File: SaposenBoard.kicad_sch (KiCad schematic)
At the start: 66 parts, among them IC1 BSO220, IC2 BSO220, IC3 BSO220, IC4 BSO220, J1 ADC4ch, J2 Extra2ch+LED, J3 Encoder1, J4 Encoder2, J5 I2C, J6 Battery, J7 Motor1, J8 Motor2, Q2 IRLML6344, SW1 BatterySW, SW2 SW_Push, SW3 SW_Push, U1 A4955GLPTR-T, U2 A4955GLPTR-T, U3 MPU-6500, U4 NUCLEO-F303K8

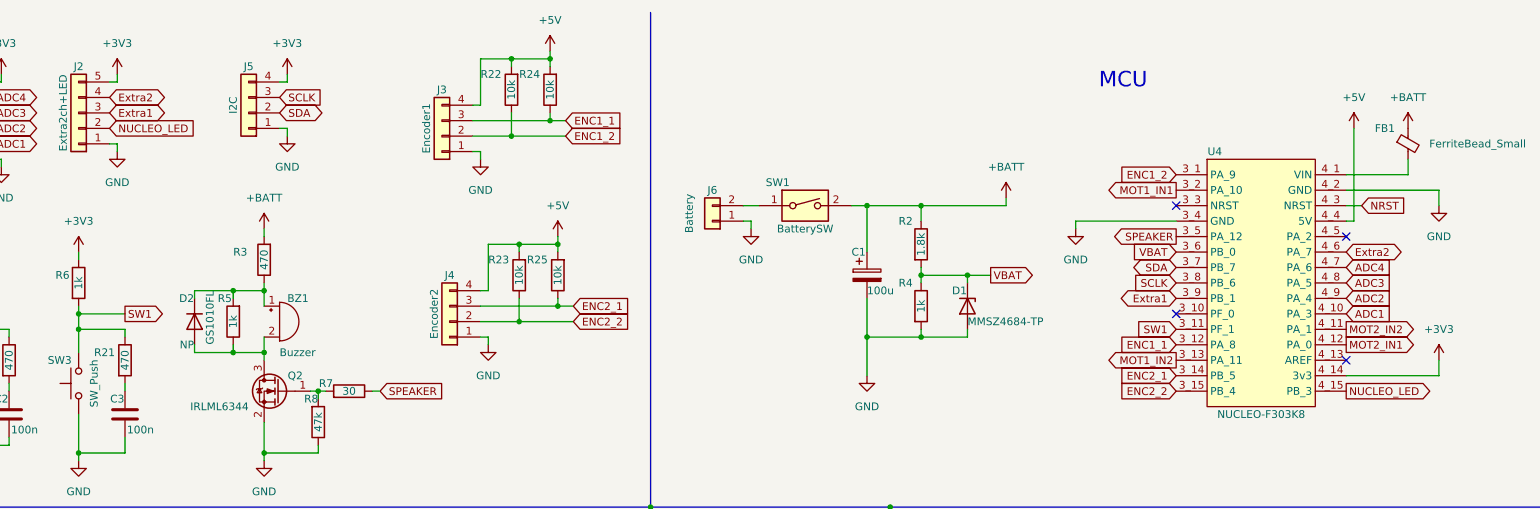
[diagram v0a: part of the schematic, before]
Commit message: [update]終わった
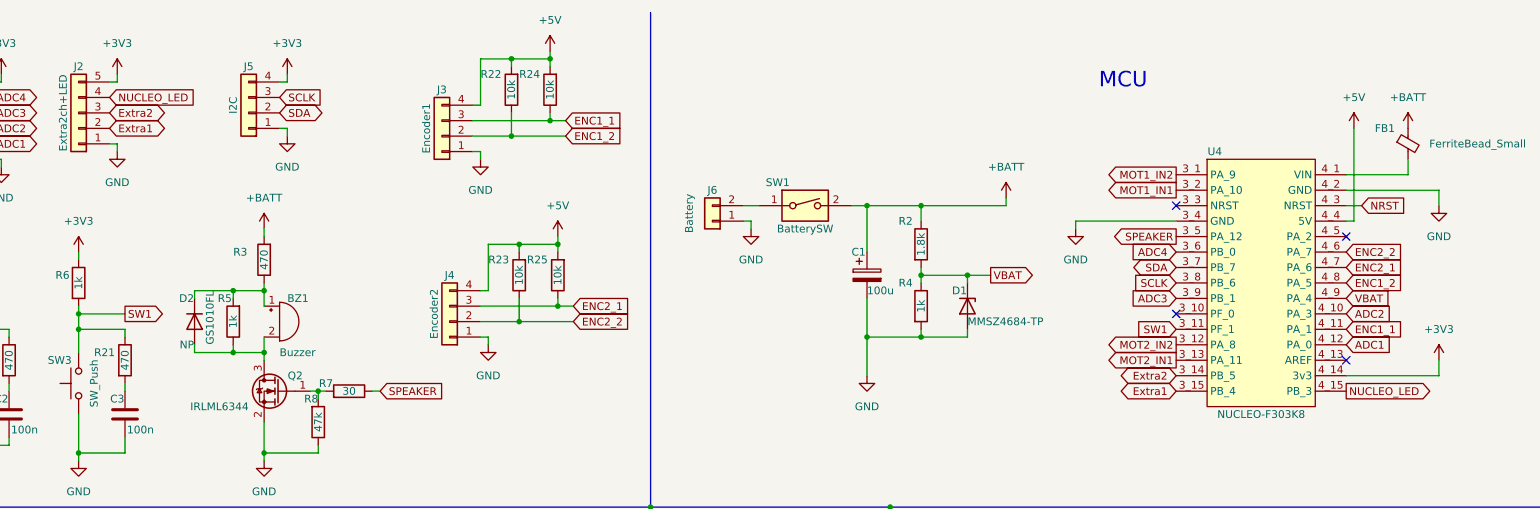
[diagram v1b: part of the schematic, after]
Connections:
- net ADC1: now also U4.4_12 (PA_0); no longer U4.4_10 (PA_3)
- net ADC2: now also U4.4_10 (PA_3); no longer U4.4_9 (PA_4)
- net ADC3: now also U4.3_9 (PB_1); no longer U4.4_8 (PA_5)
- net ADC4: now also U4.3_6 (PB_0); no longer U4.4_7 (PA_6)
- net ENC1_1: now also U4.4_11 (PA_1); no longer U4.3_12 (PA_8)
- net ENC1_2: now also U4.4_8 (PA_5); no longer U4.3_1 (PA_9)
- net ENC2_1: now also U4.4_7 (PA_6); no longer U4.3_14 (PB_5)
- net ENC2_2: now also U4.4_6 (PA_7); no longer U4.3_15 (PB_4)
- net Extra1: now also J2.2 (Pin_2), U4.3_15 (PB_4); no longer J2.3 (Pin_3), U4.3_9 (PB_1)
- net Extra2: now also J2.3 (Pin_3), U4.3_14 (PB_5); no longer J2.4 (Pin_4), U4.4_6 (PA_7)
- net MOT1_IN2: now also U4.3_1 (PA_9); no longer U4.3_13 (PA_11)
- net MOT2_IN1: now also U4.3_13 (PA_11); no longer U4.4_12 (PA_0)
- net MOT2_IN2: now also U4.3_12 (PA_8); no longer U4.4_11 (PA_1)
- net NUCLEO_LED: now also J2.4 (Pin_4); no longer J2.2 (Pin_2)
- net VBAT: now also U4.4_9 (PA_4); no longer U4.3_6 (PB_0)

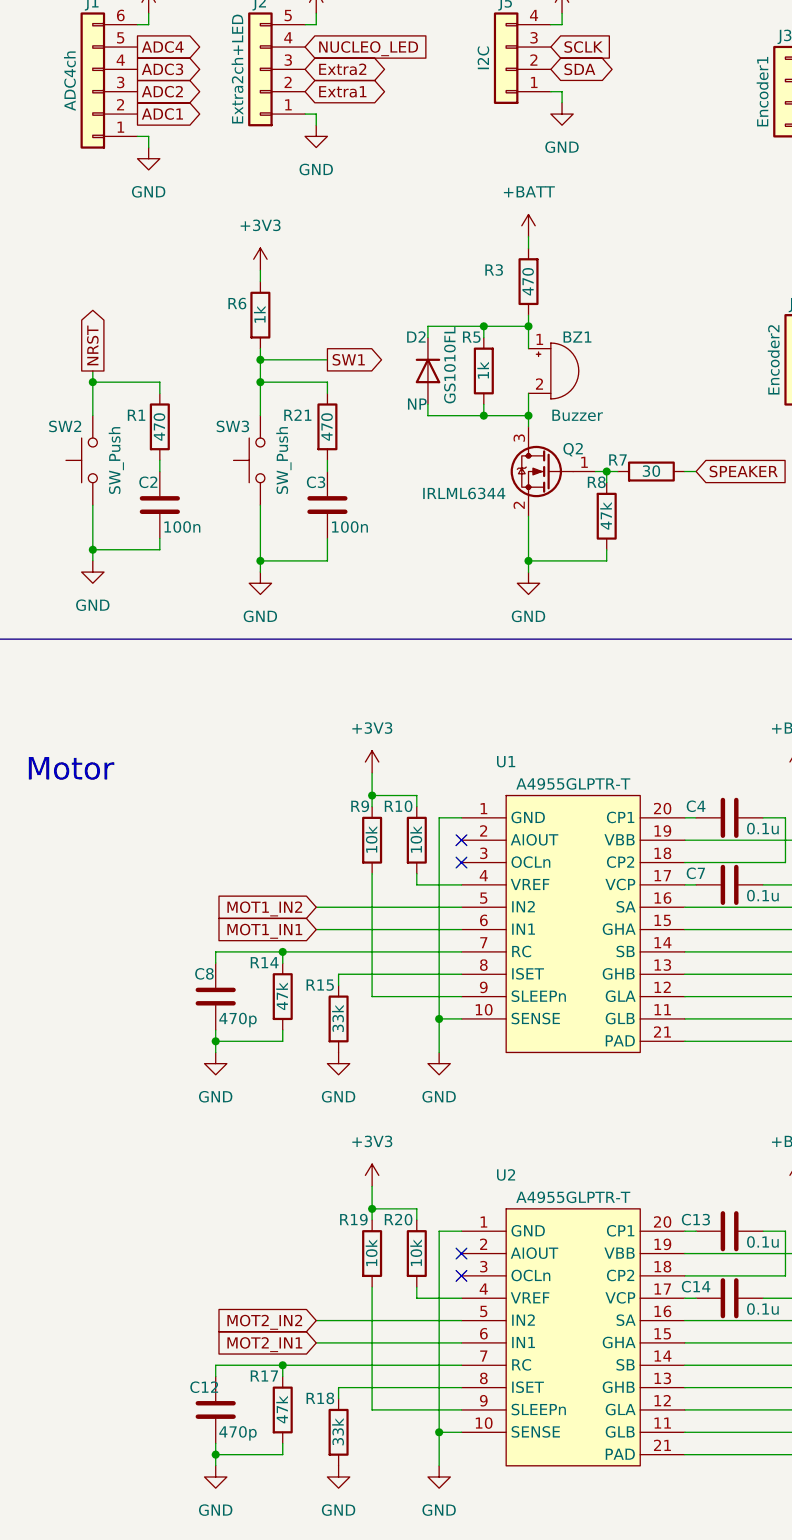
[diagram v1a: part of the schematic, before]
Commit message: a
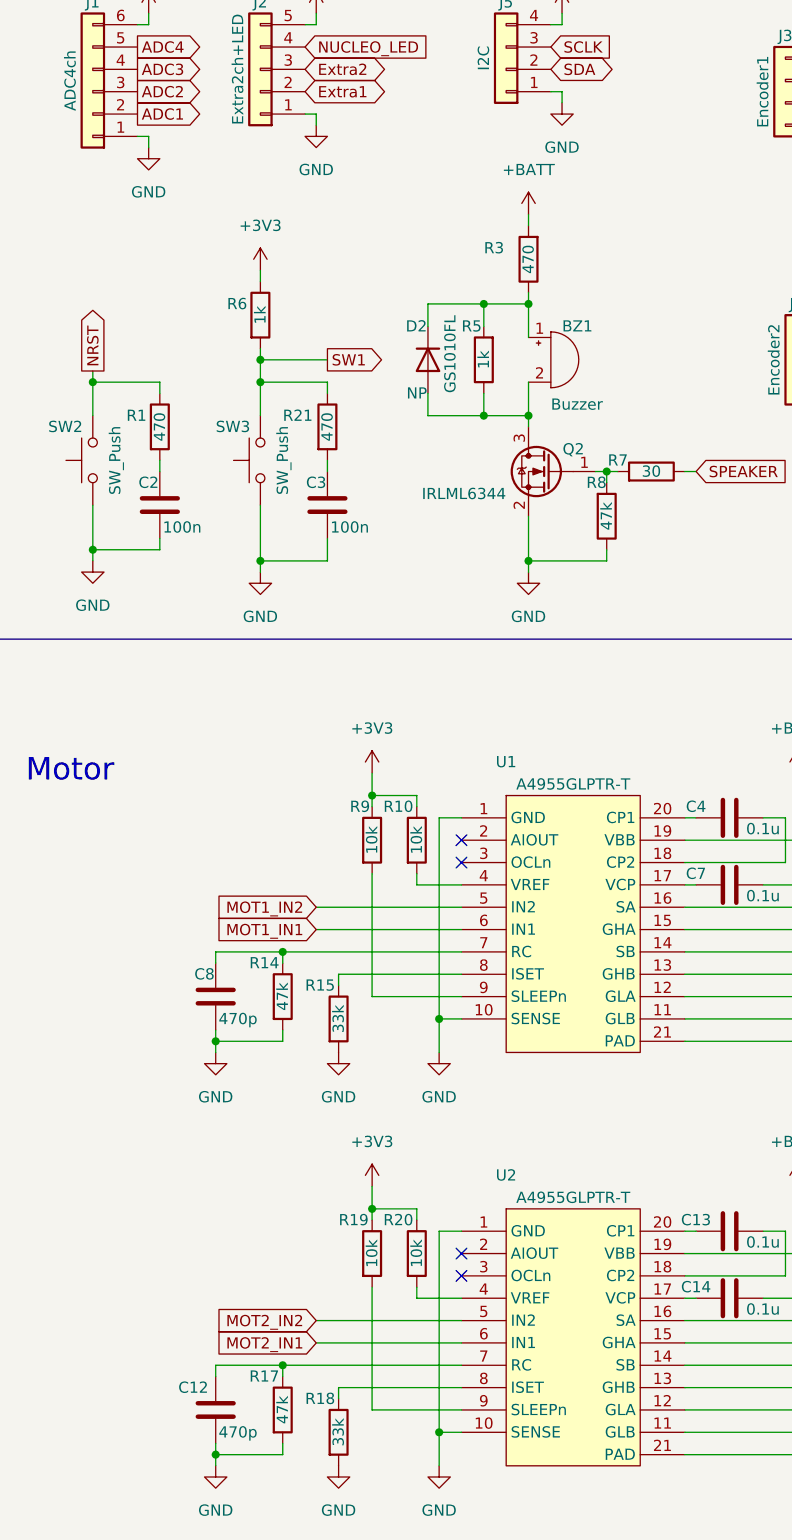
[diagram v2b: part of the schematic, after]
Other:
- moved on the sheet: BZ1, D2, R3, R5
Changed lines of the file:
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@@
   (junction (at 121.92 60.96) (diameter 0) (color 0 0 0 0)
   )
-  (junction (at 73.66 58.42) (diameter 0) (color 0 0 0 0)
+  (junction (at 73.66 55.88) (diameter 0) (color 0 0 0 0)
   )
   (junction (at 148.59 171.45) (diameter 0) (color 0 0 0 0)
@@
   (junction (at 38.1 139.7) (diameter 0) (color 0 0 0 0)
   )
+  (junction (at 68.58 55.88) (diameter 0) (color 0 0 0 0)
+  )
   (junction (at 55.88 111.76) (diameter 0) (color 0 0 0 0)
   )
@@
   )
   (junction (at 120.65 30.48) (diameter 0) (color 0 0 0 0)
-  )
-  (junction (at 68.58 58.42) (diameter 0) (color 0 0 0 0)
   )
   (junction (at 115.57 63.5) (diameter 0) (color 0 0 0 0)
@@
     (stroke (width 0) (type default) (color 0 0 0 0))
   )
-  (wire (pts (xy 62.23 67.31) (xy 62.23 68.58))
+  (wire (pts (xy 62.23 66.04) (xy 62.23 68.58))
     (stroke (width 0) (type default) (color 0 0 0 0))
   )
@@
     (stroke (width 0) (type default) (color 0 0 0 0))
   )
-  (wire (pts (xy 62.23 58.42) (xy 68.58 58.42))
+  (wire (pts (xy 62.23 55.88) (xy 68.58 55.88))
     (stroke (width 0) (type default) (color 0 0 0 0))
   )
@@
     (stroke (width 0) (type default) (color 0 0 0 0))
   )
-  (wire (pts (xy 73.66 57.15) (xy 73.66 58.42))
+  (wire (pts (xy 73.66 54.61) (xy 73.66 55.88))
     (stroke (width 0) (type default) (color 0 0 0 0))
   )
@@
     (stroke (width 0) (type default) (color 0 0 0 0))
   )
-  (wire (pts (xy 73.66 66.04) (xy 73.66 68.58))
+  (wire (pts (xy 73.66 64.77) (xy 73.66 68.58))
     (stroke (width 0) (type default) (color 0 0 0 0))
   )
@@
     (stroke (width 0) (type default) (color 0 0 0 0))
   )
+  (wire (pts (xy 68.58 55.88) (xy 68.58 58.42))
+    (stroke (width 0) (type default) (color 0 0 0 0))
+  )
   (wire (pts (xy 91.44 127) (xy 125.73 127))
     (stroke (width 0) (type default) (color 0 0 0 0))
@@
     (stroke (width 0) (type default) (color 0 0 0 0))
   )
-  (wire (pts (xy 68.58 58.42) (xy 73.66 58.42))
+  (wire (pts (xy 68.58 55.88) (xy 73.66 55.88))
     (stroke (width 0) (type default) (color 0 0 0 0))
   )
@@
     (stroke (width 0) (type default) (color 0 0 0 0))
   )
-  (wire (pts (xy 68.58 67.31) (xy 68.58 68.58))
+  (wire (pts (xy 68.58 66.04) (xy 68.58 68.58))
     (stroke (width 0) (type default) (color 0 0 0 0))
   )
@@
     (stroke (width 0) (type default) (color 0 0 0 0))
   )
-  (wire (pts (xy 73.66 58.42) (xy 73.66 60.96))
+  (wire (pts (xy 73.66 55.88) (xy 73.66 59.69))
     (stroke (width 0) (type default) (color 0 0 0 0))
   )
@@
     (stroke (width 0) (type default) (color 0 0 0 0))
   )
-  (wire (pts (xy 73.66 48.26) (xy 73.66 49.53))
+  (wire (pts (xy 73.66 45.72) (xy 73.66 46.99))
     (stroke (width 0) (type default) (color 0 0 0 0))
   )
@@
     (stroke (width 0) (type default) (color 0 0 0 0))
   )
-  (wire (pts (xy 62.23 59.69) (xy 62.23 58.42))
+  (wire (pts (xy 62.23 58.42) (xy 62.23 55.88))
     (stroke (width 0) (type default) (color 0 0 0 0))
   )
@@
   )
   (wire (pts (xy 66.04 114.3) (xy 63.5 114.3))
-    (stroke (width 0) (type default) (color 0 0 0 0))
-  )
-  (wire (pts (xy 68.58 59.69) (xy 68.58 58.42))
     (stroke (width 0) (type default) (color 0 0 0 0))
   )
@@
     (pin "1")
   )
-  (symbol (lib_id "Device:R") (at 73.66 53.34 180) (unit 1)
-    (in_bom yes) (on_board yes)
-    (property "Reference" "R3" (id 0) (at 68.58 52.07 0)
+  (symbol (lib_id "Device:R") (at 73.66 50.8 180) (unit 1)
+    (in_bom yes) (on_board yes)
+    (property "Reference" "R3" (id 0) (at 68.58 49.53 0)
       (effects (font (size 1.27 1.27)) (justify right))
     )
-    (property "Value" "470" (id 1) (at 73.66 53.34 90))
-    (property "Footprint" "Resistor_SMD:R_0603_1608Metric" (id 2) (at 75.438 53.34 90)
-      (effects (font (size 1.27 1.27)) hide)
-    )
-    (property "Datasheet" "~" (id 3) (at 73.66 53.34 0)
+    (property "Value" "470" (id 1) (at 73.66 50.8 90))
+    (property "Footprint" "Resistor_SMD:R_0603_1608Metric" (id 2) (at 75.438 50.8 90)
+      (effects (font (size 1.27 1.27)) hide)
+    )
+    (property "Datasheet" "~" (id 3) (at 73.66 50.8 0)
       (effects (font (size 1.27 1.27)) hide)
     )
@@
     (pin "2")
   )
-  (symbol (lib_id "Device:Buzzer") (at 76.2 63.5 0) (unit 1)
-    (in_bom yes) (on_board yes)
-    (property "Reference" "BZ1" (id 0) (at 77.47 59.69 0)
+  (symbol (lib_id "Device:Buzzer") (at 76.2 62.23 0) (unit 1)
+    (in_bom yes) (on_board yes)
+    (property "Reference" "BZ1" (id 0) (at 77.47 58.42 0)
       (effects (font (size 1.27 1.27)) (justify left))
     )
-    (property "Value" "Buzzer" (id 1) (at 76.2 68.58 0)
+    (property "Value" "Buzzer" (id 1) (at 76.2 67.31 0)
       (effects (font (size 1.27 1.27)) (justify left))
     )
-    (property "Footprint" "Footprints:PKM13EPYH4000-A0" (id 2) (at 75.565 60.96 90)
-      (effects (font (size 1.27 1.27)) hide)
-    )
-    (property "Datasheet" "~" (id 3) (at 75.565 60.96 90)
+    (property "Footprint" "Footprints:PKM13EPYH4000-A0" (id 2) (at 75.565 59.69 90)
+      (effects (font (size 1.27 1.27)) hide)
+    )
+    (property "Datasheet" "~" (id 3) (at 75.565 59.69 90)
       (effects (font (size 1.27 1.27)) hide)
     )
@@
     (pin "8")
   )
-  (symbol (lib_id "power:+BATT") (at 73.66 48.26 0) (unit 1)
-    (in_bom yes) (on_board yes) (fields_autoplaced)
-    (property "Reference" "#PWR015" (id 0) (at 73.66 52.07 0)
-      (effects (font (size 1.27 1.27)) hide)
-    )
-    (property "Value" "+BATT" (id 1) (at 73.66 43.18 0))
-    (property "Footprint" "" (id 2) (at 73.66 48.26 0)
-      (effects (font (size 1.27 1.27)) hide)
-    )
-    (property "Datasheet" "" (id 3) (at 73.66 48.26 0)
+  (symbol (lib_id "power:+BATT") (at 73.66 45.72 0) (unit 1)
+    (in_bom yes) (on_board yes) (fields_autoplaced)
+    (property "Reference" "#PWR015" (id 0) (at 73.66 49.53 0)
+      (effects (font (size 1.27 1.27)) hide)
+    )
+    (property "Value" "+BATT" (id 1) (at 73.66 40.64 0))
+    (property "Footprint" "" (id 2) (at 73.66 45.72 0)
+      (effects (font (size 1.27 1.27)) hide)
+    )
+    (property "Datasheet" "" (id 3) (at 73.66 45.72 0)
       (effects (font (size 1.27 1.27)) hide)
     )
@@
     (pin "1")
   )
-  (symbol (lib_id "Device:R") (at 68.58 63.5 180) (unit 1)
-    (in_bom yes) (on_board yes)
-    (property "Reference" "R5" (id 0) (at 66.04 59.69 0)
+  (symbol (lib_id "Device:R") (at 68.58 62.23 180) (unit 1)
+    (in_bom yes) (on_board yes)
+    (property "Reference" "R5" (id 0) (at 66.04 58.42 0)
       (effects (font (size 1.27 1.27)) (justify right))
     )
-    (property "Value" "1k" (id 1) (at 68.58 63.5 90))
-    (property "Footprint" "Resistor_SMD:R_0603_1608Metric" (id 2) (at 70.358 63.5 90)
-      (effects (font (size 1.27 1.27)) hide)
-    )
-    (property "Datasheet" "~" (id 3) (at 68.58 63.5 0)
+    (property "Value" "1k" (id 1) (at 68.58 62.23 90))
+    (property "Footprint" "Resistor_SMD:R_0603_1608Metric" (id 2) (at 70.358 62.23 90)
+      (effects (font (size 1.27 1.27)) hide)
+    )
+    (property "Datasheet" "~" (id 3) (at 68.58 62.23 0)
       (effects (font (size 1.27 1.27)) hide)
     )
@@
   (symbol (lib_id "Device:C") (at 38.1 181.61 0) (unit 1)
     (in_bom yes) (on_board yes)
-    (property "Reference" "C12" (id 0) (at 36.83 179.07 0))
+    (property "Reference" "C12" (id 0) (at 35.56 179.07 0))
     (property "Value" "470p" (id 1) (at 40.64 184.15 0))
     (property "Footprint" "Capacitor_SMD:C_0603_1608Metric" (id 2) (at 39.0652 185.42 0)
@@
     (pin "1")
   )
-  (symbol (lib_id "Device:D") (at 62.23 63.5 270) (unit 1)
-    (in_bom yes) (on_board yes)
-    (property "Reference" "D2" (id 0) (at 59.69 59.69 90)
+  (symbol (lib_id "Device:D") (at 62.23 62.23 270) (unit 1)
+    (in_bom yes) (on_board yes)
+    (property "Reference" "D2" (id 0) (at 59.69 58.42 90)
       (effects (font (size 1.27 1.27)) (justify left))
     )
-    (property "Value" "GS1010FL" (id 1) (at 64.77 58.42 0)
+    (property "Value" "GS1010FL" (id 1) (at 64.77 57.15 0)
       (effects (font (size 1.27 1.27)) (justify left))
     )
-    (property "Footprint" "Diode_SMD:D_SOD-123F" (id 2) (at 62.23 63.5 0)
-      (effects (font (size 1.27 1.27)) hide)
-    )
-    (property "Datasheet" "~" (id 3) (at 62.23 63.5 0)
-      (effects (font (size 1.27 1.27)) hide)
-    )
-    (property "Field4" "NP" (id 4) (at 60.96 67.31 90))
-    (pin "1")
-    (pin "2")
+    (property "Footprint" "Diode_SMD:D_SOD-123F" (id 2) (at 62.23 62.23 0)
+      (effects (font (size 1.27 1.27)) hide)
+    )
+    (property "Datasheet" "~" (id 3) (at 62.23 62.23 0)
+      (effects (font (size 1.27 1.27)) hide)
+    )
+    (property "Field4" "NP" (id 4) (at 60.96 66.04 90))
+    (pin "1")
+    (pin "2")
